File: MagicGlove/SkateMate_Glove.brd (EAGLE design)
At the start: 40.9 x 27.1 mm, 45 parts, among them IC1 BU33TD3WG, IC2 LMV321M5, U2 ATMEGA328PB-AU

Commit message: Receiver Board v1.0 working
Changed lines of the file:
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@@
 <wire x1="21.04" y1="2.79" x2="22.725703125" y2="1.104296875" width="0.3048" layer="16"/>
 <wire x1="21.04" y1="2.79" x2="20.7525" y2="3.0775" width="0.3048" layer="16"/>
-<wire x1="32.39" y1="9.9855" x2="32.39" y2="15.68" width="0.3048" layer="16"/>
-<wire x1="32.39" y1="9.9855" x2="32.4055" y2="9.97" width="0.3048" layer="16"/>
+<wire x1="32.39" y1="12.36" x2="32.39" y2="15.68" width="0.3048" layer="16"/>
 <wire x1="33.7591" y1="17.2673" x2="33.7591" y2="16.315" width="0.3048" layer="1"/>
 <wire x1="33.7591" y1="17.0491" x2="33.7591" y2="17.2673" width="0.3048" layer="16"/>
@@
 <wire x1="14.165" y1="14.22" x2="14.165" y2="15.4237" width="0.3048" layer="16"/>
 <wire x1="14.165" y1="15.4237" x2="14.1415" y2="15.4472" width="0.3048" layer="16"/>
-<wire x1="32.4055" y1="9.97" x2="32.79" y2="12.26" width="0" layer="19" extent="1-1"/>
+<wire x1="32.39" y1="9.97" x2="32.4055" y2="9.97" width="0.4064" layer="16"/>
+<wire x1="32.4055" y1="9.97" x2="32.39" y2="9.97" width="0.3048" layer="16"/>
+<wire x1="32.39" y1="9.97" x2="32.39" y2="12.36" width="0.3048" layer="16"/>
 </signal>
 <signal name="RESETICSP">

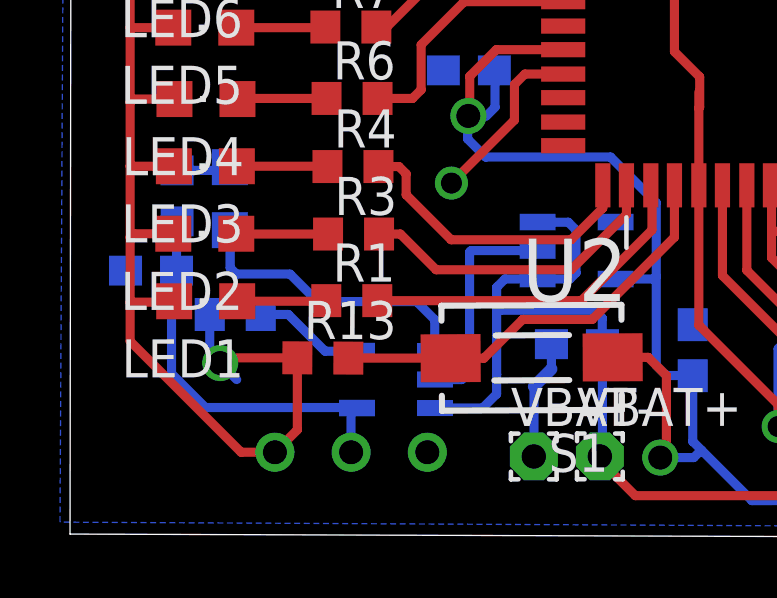
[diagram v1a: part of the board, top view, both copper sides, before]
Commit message: style
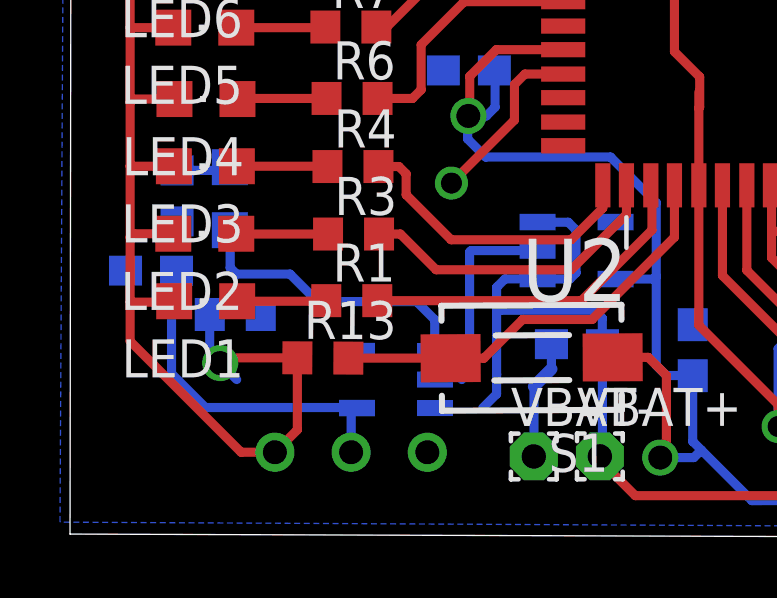
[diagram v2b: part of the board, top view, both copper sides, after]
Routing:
- net N$5: track 3.73 -> 0.00 mm
- net N$24: track 13.4 -> 11.5 mm
- net VBAT+: track 62.2 -> 60.6 mm
- net GND: track 92.7 -> 91.9 mm
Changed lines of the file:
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@@
 <?xml version="1.0" encoding="utf-8"?>
 <!DOCTYPE eagle SYSTEM "eagle.dtd">
-<eagle version="8.1.0">
+<eagle version="7.6.0">
 <drawing>
 <settings>
@@
 <contactref element="C9" pad="2"/>
 <contactref element="R11" pad="2"/>
-<contactref element="U$1" pad="2"/>
 <contactref element="VBAT-" pad="1"/>
 <polygon width="0.3048" layer="16" spacing="0.254" isolate="0.6096">
@@
 <wire x1="13.366" y1="9.44" x2="15.5824" y2="9.44" width="0.3048" layer="16"/>
 <wire x1="13.366" y1="9.44" x2="13.3145" y2="9.3885" width="0.3048" layer="16"/>
-<wire x1="12.1625" y1="5.14" x2="13.0535" y2="5.14" width="0.3048" layer="16"/>
 <wire x1="13.0535" y1="5.14" x2="13.3145" y2="5.401" width="0.3048" layer="16"/>
 <wire x1="13.3145" y1="5.401" x2="13.3145" y2="9.3885" width="0.3048" layer="16"/>
@@
 <wire x1="2" y1="6.4175" x2="5.7" y2="2.7175" width="0.3048" layer="1"/>
 <wire x1="2" y1="7.72" x2="2" y2="6.4175" width="0.3048" layer="1"/>
-<wire x1="3.4365" y1="7.72" x2="3.4675" y2="7.751" width="0" layer="19" extent="1-1"/>
+<contactref element="U$1" pad="2"/>
+<wire x1="37.33" y1="15.16" x2="37.3537" y2="16.0566" width="0" layer="19" extent="1-16"/>
+<wire x1="31.12" y1="16.16" x2="31.47" y2="18.54" width="0" layer="19" extent="1-16"/>
+<wire x1="29.6544" y1="21.1544" x2="31.36" y2="18.65" width="0" layer="19" extent="1-16"/>
+<wire x1="24.88" y1="19.9" x2="26.3656" y2="21.1544" width="0" layer="19" extent="1-1"/>
+<wire x1="16.4352" y1="15.3236" x2="24.6648" y2="16.1364" width="0" layer="19" extent="1-1"/>
+<wire x1="13.366" y1="9.44" x2="12.71" y2="11.69" width="0" layer="19" extent="1-16"/>
+<wire x1="12.1625" y1="5.14" x2="13.0535" y2="5.14" width="0" layer="19" extent="16-16"/>
+<wire x1="15.46" y1="4.91" x2="13.3145" y2="5.401" width="0" layer="19" extent="16-16"/>
+<wire x1="12.4415" y1="15.4472" x2="14.81" y2="14.975" width="0" layer="19" extent="1-16"/>
+<wire x1="11.906" y1="2.7175" x2="12.1625" y2="5.14" width="0" layer="19" extent="16-16"/>
+<wire x1="7.574209375" y1="3.465709375" x2="11.906" y2="2.7175" width="0" layer="19" extent="1-1"/>
+<wire x1="3.4675" y1="7.751" x2="3.4365" y2="7.72" width="0" layer="19" extent="1-1"/>
+<wire x1="1.8465" y1="8.7701" x2="2" y2="7.72" width="0" layer="19" extent="1-16"/>
+<wire x1="20.7525" y1="6.97" x2="16.0425" y2="6.32" width="0" layer="19" extent="16-16"/>
+<wire x1="32.4055" y1="4.89" x2="31.856" y2="14.368" width="0" layer="19" extent="1-1"/>
 </signal>
 <signal name="+3V3">
@@
 <contactref element="C8" pad="1"/>
 <contactref element="IC1" pad="3"/>
-<contactref element="U$1" pad="3"/>
 <contactref element="VBAT+" pad="1"/>
 <wire x1="14.3225" y1="7.45" x2="14.3325" y2="7.44" width="0.3048" layer="16"/>
 <wire x1="15.5789" y1="8.4865" x2="15.5824" y2="8.49" width="0.3048" layer="16"/>
-<wire x1="12.17" y1="4.1975" x2="12.1625" y2="4.19" width="0.3048" layer="16"/>
-<wire x1="12.1625" y1="4.19" x2="13.7485" y2="4.19" width="0.3048" layer="16"/>
 <wire x1="13.7485" y1="4.19" x2="14.2155" y2="4.657" width="0.3048" layer="16"/>
 <wire x1="14.2155" y1="4.657" x2="14.2155" y2="5.313" width="0.3048" layer="16"/>
@@
 <wire x1="37.86" y1="17.89" x2="38.08" y2="17.89" width="0.3048" layer="1"/>
 <wire x1="38.08" y1="17.89" x2="39.473628125" y2="16.496371875" width="0.3048" layer="1"/>
+<contactref element="U$1" pad="3"/>
+<wire x1="12.1625" y1="4.19" x2="13.7485" y2="4.19" width="0" layer="19" extent="16-16"/>
 </signal>
 <signal name="N$22">
@@
 <contactref element="U$1" pad="4"/>
 <contactref element="R12" pad="1"/>
-<contactref element="C9" pad="1"/>
 <contactref element="U$3" pad="P$1"/>
 <wire x1="9.366" y1="2.7175" x2="9.366" y2="3.9935" width="0.3048" layer="16"/>
@@
 <wire x1="9.544" y1="4.2085" x2="9.5625" y2="4.19" width="0.3048" layer="16"/>
 <wire x1="3.38" y1="5.3345" x2="3.38" y2="8.6036" width="0.3048" layer="16"/>
-<wire x1="3.38" y1="8.6036" x2="3.5465" y2="8.7701" width="0.3048" layer="16"/>
-<wire x1="3.5465" y1="8.7701" x2="3.5465" y2="10.3948" width="0.3048" layer="16"/>
 <wire x1="3.5465" y1="10.3948" x2="3.566" y2="10.4143" width="0.3048" layer="16"/>
-</signal>
-<signal name="N$25">
-<contactref element="U$1" pad="5"/>
-<contactref element="R11" pad="1"/>
-<wire x1="9.5625" y1="6.09" x2="9.5525" y2="6.1" width="0.3048" layer="16"/>
-<wire x1="6.3525" y1="7.31" x2="7.273" y2="7.31" width="0.3048" layer="16"/>
-<wire x1="7.273" y1="7.31" x2="8.496" y2="6.087" width="0.3048" layer="16"/>
-<wire x1="8.496" y1="6.087" x2="9.5595" y2="6.087" width="0.3048" layer="16"/>
-<wire x1="9.5595" y1="6.087" x2="9.5625" y2="6.09" width="0.3048" layer="16"/>
+<contactref element="C9" pad="1"/>
+<wire x1="3.5465" y1="8.7701" x2="3.5465" y2="10.3948" width="0" layer="19" extent="16-16"/>
+<wire x1="3.38" y1="8.6036" x2="3.5465" y2="8.7701" width="0" layer="19" extent="16-16"/>
 </signal>
 <signal name="N$3">
@@
 <wire x1="28.0844" y1="18.4544" x2="28.99" y2="19.36" width="0.3048" layer="1"/>
 </signal>
+<signal name="N$5">
+<contactref element="U$1" pad="5"/>
+<contactref element="R11" pad="1"/>
+<wire x1="6.3525" y1="7.31" x2="9.5625" y2="6.09" width="0" layer="19" extent="16-16"/>
+</signal>
 </signals>
